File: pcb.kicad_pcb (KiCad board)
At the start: 4 copper layers, 32 x 47 mm, 63 parts, among them J1 USB_C_Receptacle_USB2.0, J2 OLED, Q1 2N7002, Q2 Si2301CDS, Q3 2N7002, Q4 Si2301CDS, SW1 SW_Push, U1 ADXL375, U2 ESP32-S3-MINI-1, U3 AMS1117-3.3, U4 MCP73831-2-OT, U5 W25Q128JVS

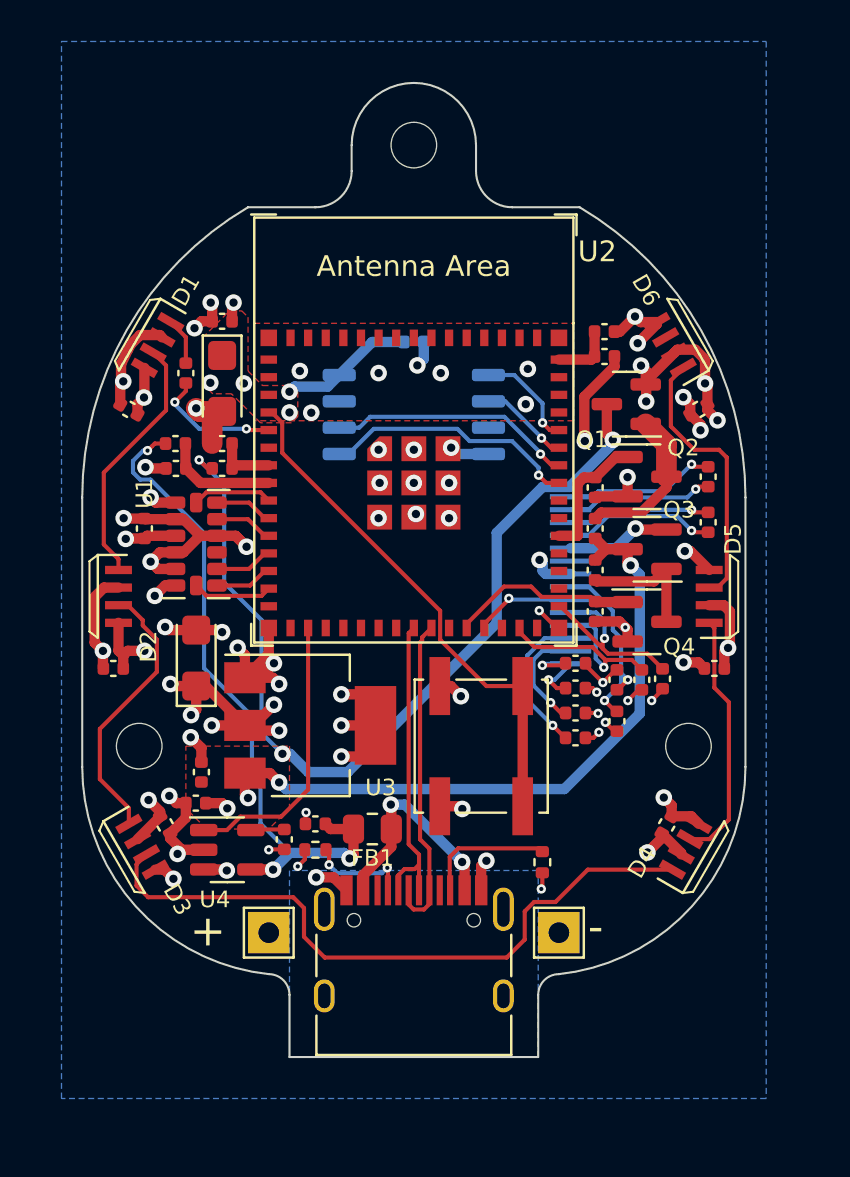
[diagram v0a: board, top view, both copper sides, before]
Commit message: added part numbers
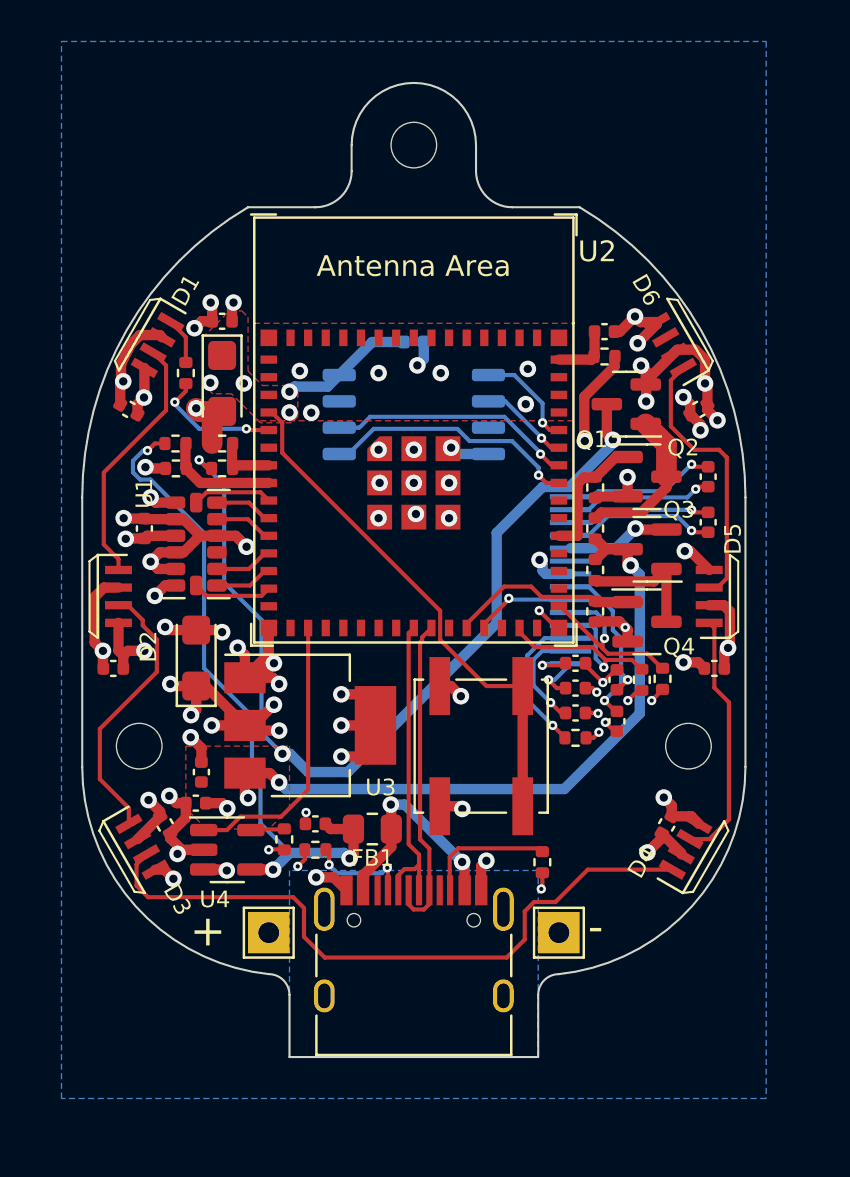
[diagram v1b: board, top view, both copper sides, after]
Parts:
- R1, R10, R11, R12, R15, R16, R17, R18, R2, R3, R4, R5, R8, R9: footprint Capacitor_SMD:C_0402_1005Metric -> Resistor_SMD:R_0402_1005Metric

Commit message: Bare ESP layout
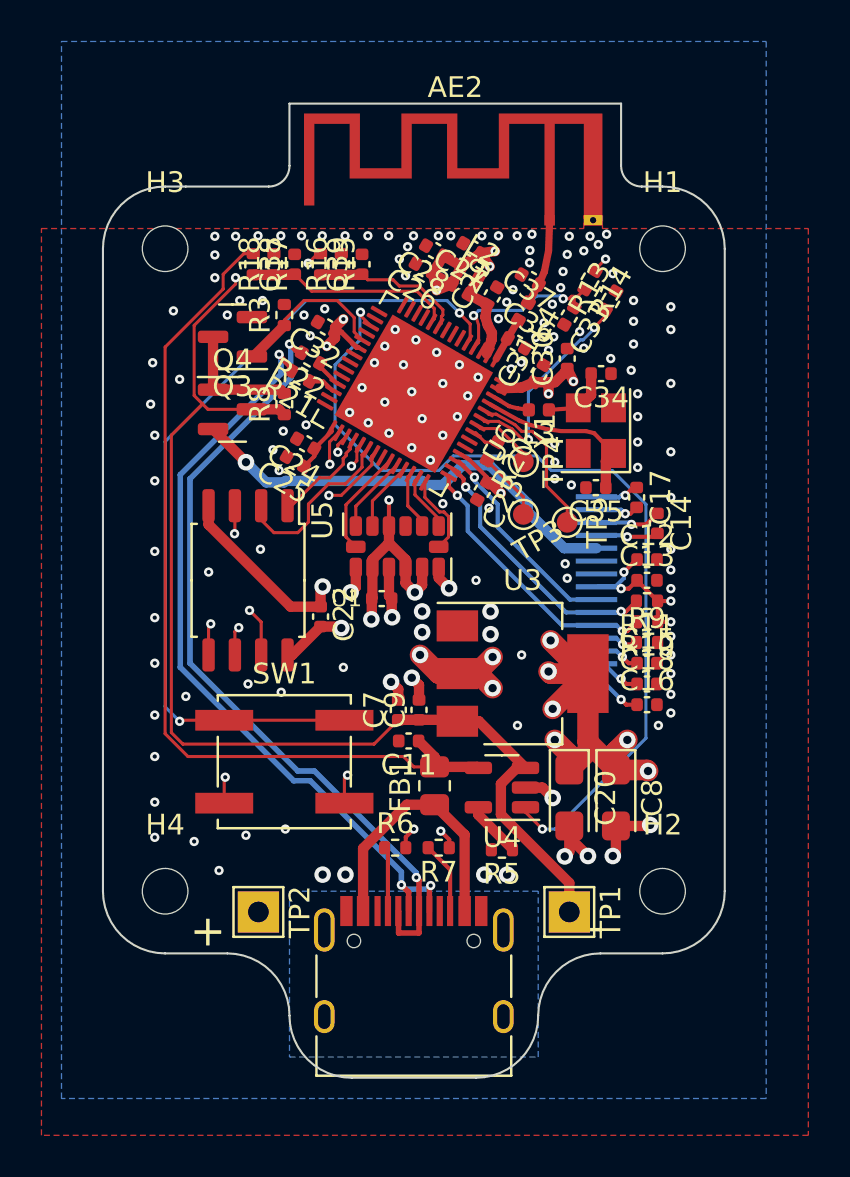
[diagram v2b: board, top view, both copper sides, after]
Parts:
- removed C1, C2, C21, C3, C4, C5, C6: 100n, Capacitor_SMD:C_0402_1005Metric
- removed C19: 1u, Capacitor_SMD:C_0402_1005Metric
- removed D1, D2, D3, D4, D5, D6: WS2812B-4020, WS2812B-4020:WS2812B-4020
- removed Q1: 2N7002, Package_TO_SOT_SMD:SOT-23
- removed Q2: Si2301CDS, Package_TO_SOT_SMD:SOT-23
- removed R1, R12, R2: 10k, Resistor_SMD:R_0402_1005Metric
- removed R4: 100, Resistor_SMD:R_0402_1005Metric
- removed U2: ESP32-S3-MINI-1, Espressif:ESP32-S3-MINI-1
- added AE2: PCB Antenna, RF_Antenna:Texas_SWRA117D_2.4GHz_Left, F.Cu at (165.6, 58.6)
- added C23: 100n, Capacitor_SMD:C_0402_1005Metric, F.Cu at (162.3, 71.7)
- added C24: 100n, Capacitor_SMD:C_0402_1005Metric, F.Cu at (153.8, 69.4)
- added C25: 1u, Capacitor_SMD:C_0402_1005Metric, F.Cu at (153.3, 70.3)
- added C26: 100n, Capacitor_SMD:C_0402_1005Metric, F.Cu at (159.5, 61.0)
- added C27: 1u, Capacitor_SMD:C_0402_1005Metric, F.Cu at (161.8, 60.0)
- added C28: 10u, Capacitor_SMD:C_0402_1005Metric, F.Cu at (160.0, 60.1)
- added C29: 100n, Capacitor_SMD:C_0402_1005Metric, F.Cu at (162.8, 62.3)
- added C30: 10u, Capacitor_SMD:C_0402_1005Metric, F.Cu at (166.4, 65.3)
- added C31: 1u, Capacitor_SMD:C_0402_1005Metric, F.Cu at (165.0, 66.0)
- added C32: 100n, Capacitor_SMD:C_0402_1005Metric, F.Cu at (154.8, 63.8)
- added C33: 1u, Capacitor_SMD:C_0402_1005Metric, F.Cu at (166.5, 63.2)
- added C34: 22p, Capacitor_SMD:C_0402_1005Metric, F.Cu at (168.0, 66.0)
- added C35: 22p, Capacitor_SMD:C_0402_1005Metric, F.Cu at (167.8, 71.5)
- added C36: 4p7, Capacitor_SMD:C_0402_1005Metric, F.Cu at (163.9, 64.6)
- added C37: 3p3, Capacitor_SMD:C_0402_1005Metric, F.Cu at (164.6, 61.5)
- added C38: 100n, Capacitor_SMD:C_0402_1005Metric, F.Cu at (153.2, 60.8)
- added C39: 100n, Capacitor_SMD:C_0402_1005Metric, F.Cu at (156.5, 60.8)
- added H4: MountingHole, MountingHole:MountingHole_2.2mm_M2, F.Cu at (147.0, 91.0)
- added L1: 3.9nH, Inductor_SMD:L_0402_1005Metric, F.Cu at (161.2, 62.0)
- added L2: 3.9nH, Inductor_SMD:L_0402_1005Metric, F.Cu at (161.7, 61.1)
- added L3: 15nH, Inductor_SMD:L_0402_1005Metric, F.Cu at (165.0, 67.8)
- added L4: 1.8nH, Inductor_SMD:L_0402_1005Metric, F.Cu at (164.3, 63.0)
- added R13: 10k, Resistor_SMD:R_0402_1005Metric, F.Cu at (168.5, 62.5)
- added R14: 10k, Resistor_SMD:R_0402_1005Metric, F.Cu at (167.5, 61.5)
- added R20: 470, Resistor_SMD:R_0402_1005Metric, F.Cu at (162.8, 69.8)
- added R21: 0R, Resistor_SMD:R_0402_1005Metric, F.Cu at (153.5, 66.1)
- added R22: 0R, Resistor_SMD:R_0402_1005Metric, F.Cu at (154.0, 65.3)
- added TP3: TXD, TestPoint:TestPoint_Pad_D1.0mm, F.Cu at (164.3, 72.8)
- added TP4: RXD, TestPoint:TestPoint_Pad_D1.0mm, F.Cu at (164.3, 70.3)
- added TP5: BOOT1, TestPoint:TestPoint_Pad_D1.0mm, F.Cu at (166.4, 73.2)
- added U6: ESP32-S3, Package_DFN_QFN:QFN-56-1EP_7x7mm_P0.4mm_EP5.6x5.6mm, F.Cu at (159.0, 67.0)
- added Y1: 40MHz 15pF, Crystal:Crystal_SMD_3225-4Pin_3.2x2.5mm, F.Cu at (167.8, 68.8)
- C22, U5: moved to F.Cu
- R10, R11: value 4k7 -> 10k
- R15, R16, R17, R18: value 100k -> 120k
- moved H2 26.2 mm to (171.0, 91.0)
- moved C20 26.1 mm to (166.5, 86.5)
- moved Q3 24.3 mm to (150.2, 64.2), turned to 180 degrees
- moved H1 24.0 mm to (171.0, 60.0)
- moved C8 21.3 mm to (168.8, 86.5), turned to -90 degrees
- moved Q4 21.1 mm to (150.2, 67.8), turned to 0 degrees
- moved R3 20.7 mm to (152.8, 63.2), turned to 90 degrees
- moved R8 17.0 mm to (152.8, 67.5), turned to 90 degrees
- moved TP1 14.5 mm to (166.5, 92.0), turned to -90 degrees
- moved TP2 14.5 mm to (151.5, 92.0), turned to -90 degrees
- moved C22 14.0 mm to (154.5, 77.8), turned to 90 degrees
- moved U4 13.6 mm to (163.2, 86.0), turned to 180 degrees
- moved H3 13.0 mm to (147.0, 60.0)
- moved C10 11.9 mm to (157.4, 76.9), turned to 180 degrees
- moved C9 11.7 mm to (159.2, 82.2), turned to 90 degrees
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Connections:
- U5 pad 2: FLASH-SDO -> FLASH-Q
- U5 pad 3: unconnected-(U5-IO2-Pad3) -> FLASH-WP
- U5 pad 5: FLASH-SDI -> FLASH-D
- U5 pad 6: FLASH-SCK -> FLASH-CLK
- U5 pad 7: unconnected-(U5-IO3-Pad7) -> FLASH-HD
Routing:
- net GND: track 78.2 -> 34.3 mm, vias 58 -> 155
- net Net-(D3-DOUT): track 32.4 -> 0.00 mm
- net CHARGE_STAT: track 13.6 -> 43.5 mm, vias 0 -> 2
- net /LEDs/VLED: track 27.8 -> 0.00 mm, vias 9 -> 0
- net VBAT: track 86.6 -> 60.1 mm, vias 8 -> 2
- net USB_D-: track 14.9 -> 38.3 mm, vias 0 -> 2
- net USB_D+: track 15.6 -> 37.8 mm, vias 0 -> 3
- net +3.3V: track 46.1 -> 64.7 mm, vias 21 -> 26
- net /OLED/OLED-VBAT: track 5.04 -> 22.0 mm
- net /BOOT: track 25.2 -> 40.7 mm, vias 0 -> 2
- net FLASH-D: track 0.00 -> 13.4 mm, vias 0 -> 2
- net Net-(D2-DOUT): track 13.3 -> 0.00 mm
- net Net-(D5-DOUT): track 13.3 -> 0.00 mm
- net FLASH-HD: track 0.00 -> 13.2 mm, vias 0 -> 2
- net FLASH-CLK: track 0.00 -> 12.9 mm, vias 0 -> 2
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- removed copper zone on F.Cu, net +3.3V
- removed copper zone on In2.Cu, net /LEDs/VLED
- removed copper zone on F.Cu, net VBAT
- removed copper zone on In2.Cu, net VBAT
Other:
- board size 32 x 47 mm -> 30 x 47 mm
